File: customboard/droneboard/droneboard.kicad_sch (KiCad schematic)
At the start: 49 parts, among them J1 Conn_01x04, J2 USB_B_Micro, J3 Conn_01x05_Pin, J4 Conn_01x02_Pin, SW1 SW_Push, SW2 SW_Push, U1 STM32F411CEUx, U3 L78M05CDT, U4 ICM-42688-P, U5 LDK130M33R, U6 LDK130M33R, Y2 CSTNE20M0V53Z000R0

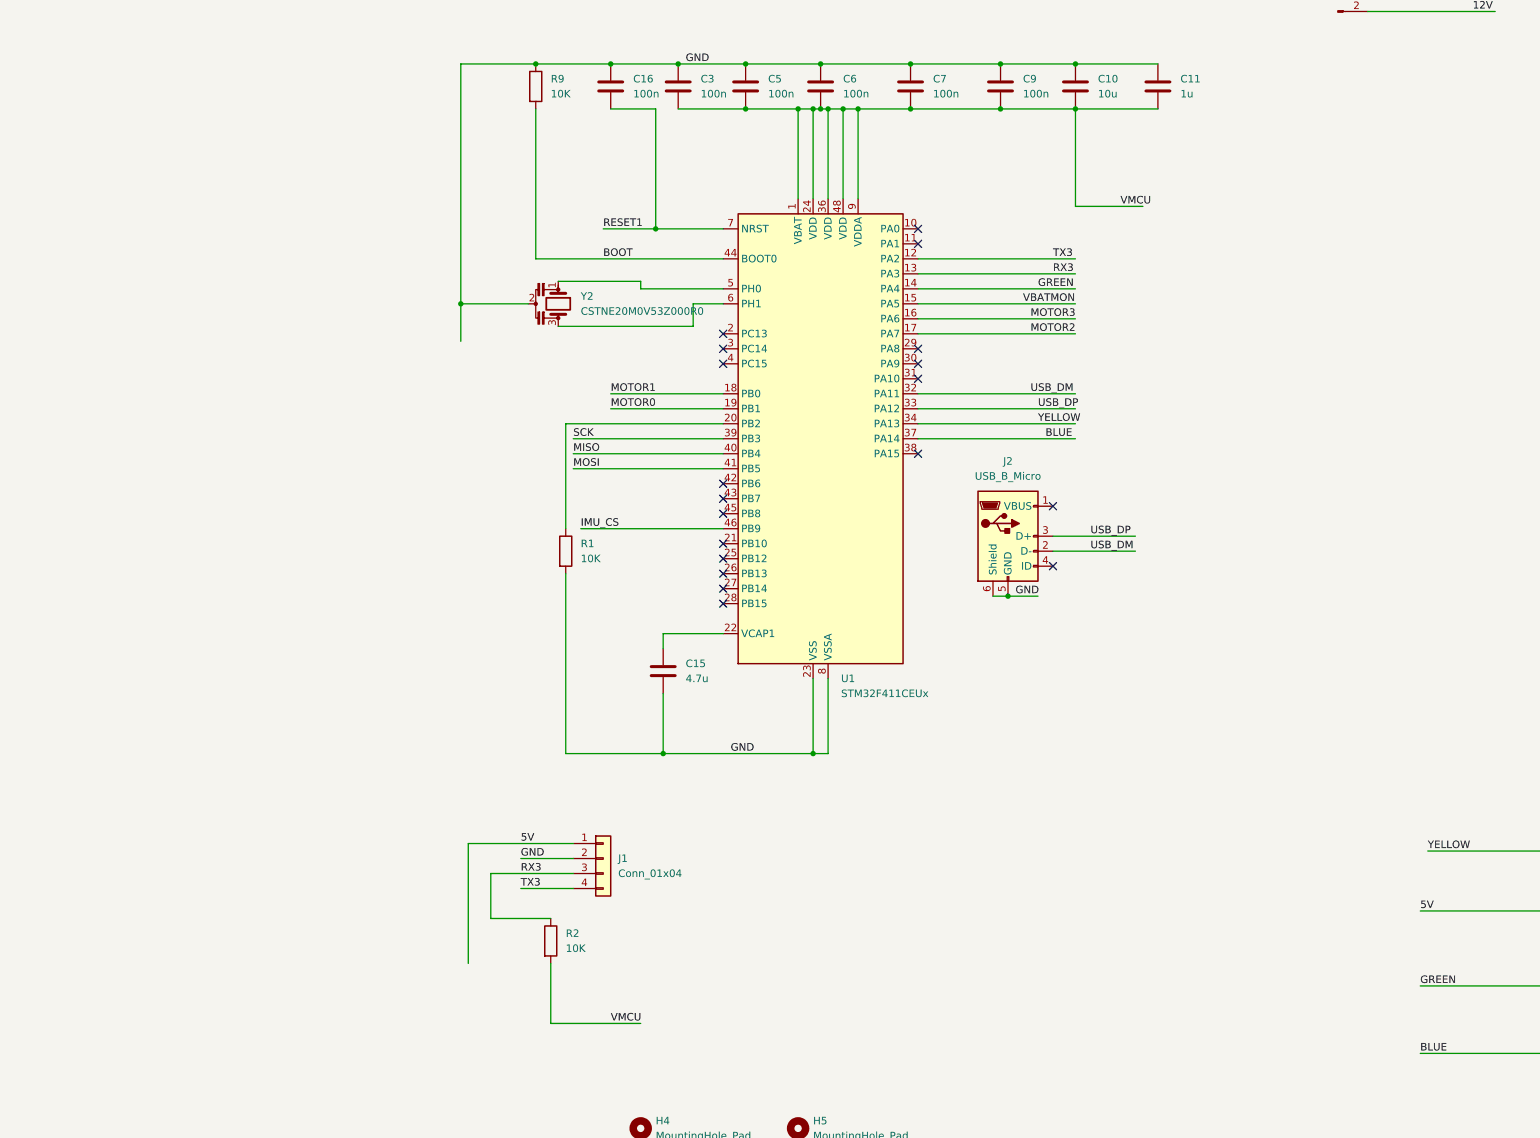
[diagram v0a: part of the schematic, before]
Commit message: h7 initial
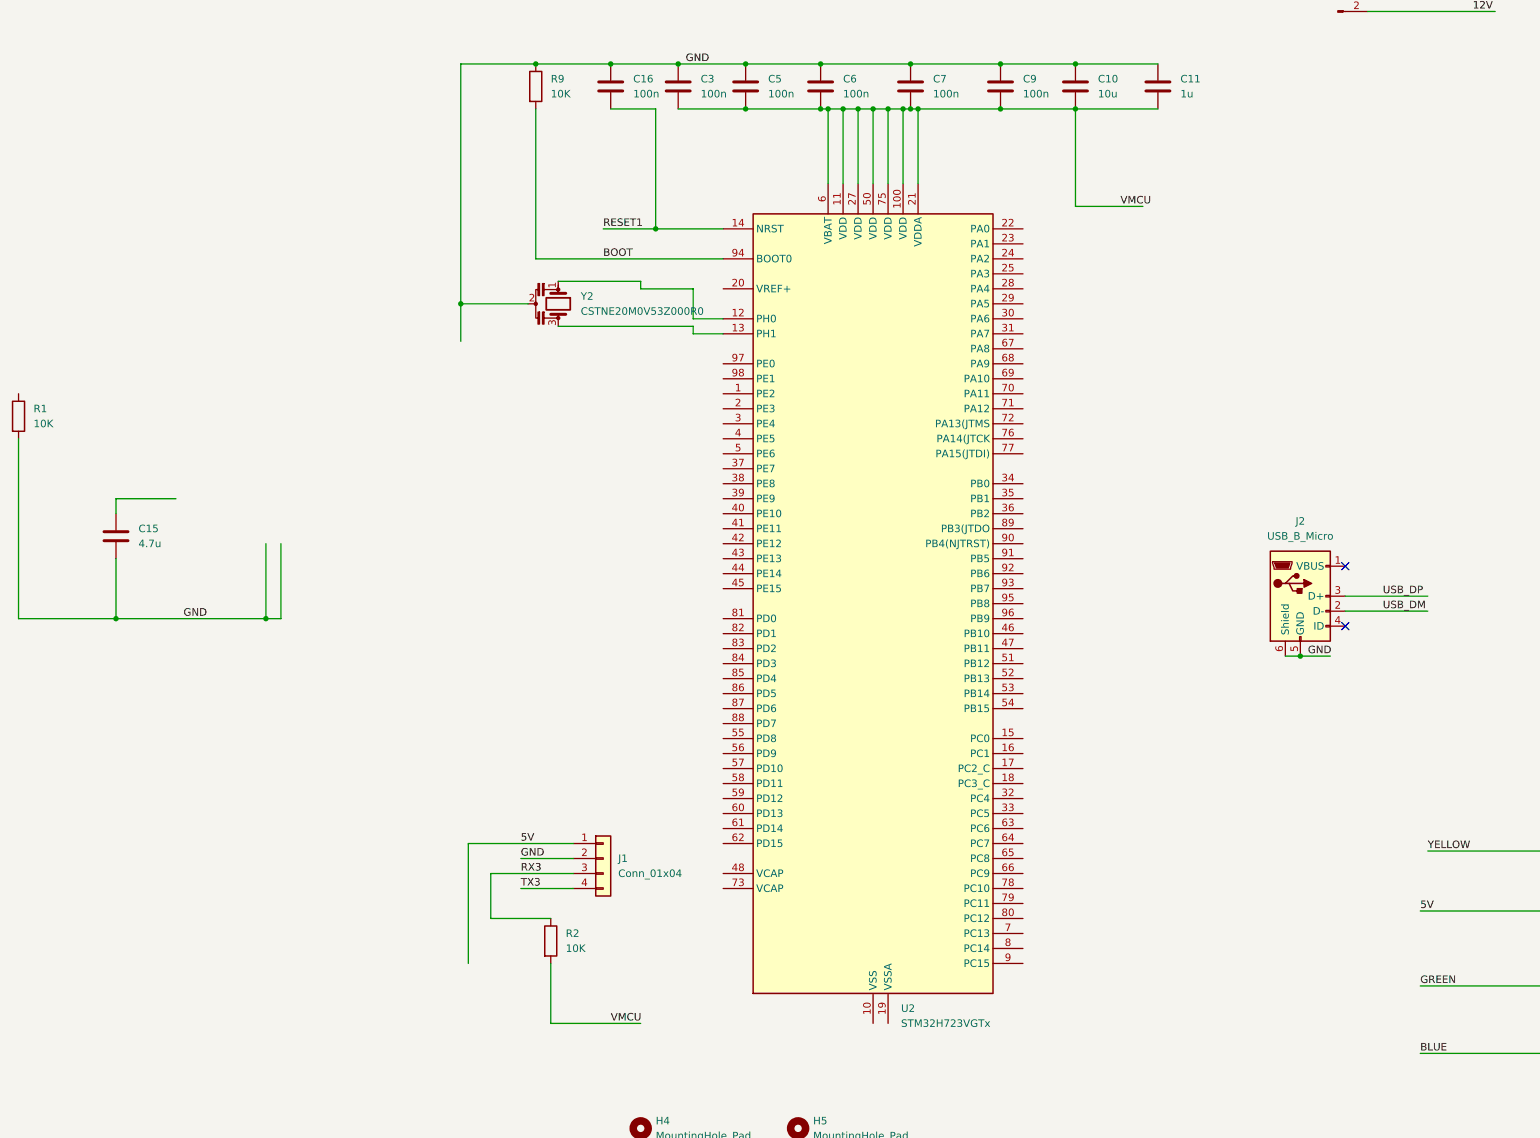
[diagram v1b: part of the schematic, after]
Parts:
- removed U1: STM32F411CEUx, Package_DFN_QFN:QFN-48-1EP_7x7mm_P0.5mm_EP5.6x5.6mm, symbol MCU_ST_STM32F4:STM32F411CEUx
- added U2: STM32H723VGTx, Package_QFP:LQFP-100_14x14mm_P0.5mm, symbol MCU_ST_STM32H7:STM32H723VGTx
- J4: footprint Connector_JST:JST_XH_B2B-XH-A_1x02_P2.50mm_Vertical -> Connector_PinHeader_1.27mm:PinHeader_1x02_P1.27mm_Vertical
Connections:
- net BOOT: now also U2.94 (BOOT0)
- net RESET1: now also U2.14 (NRST)
- net VMCU: now also U2.100 (VDD), U2.11 (VDD), U2.21 (VDDA), U2.27 (VDD), U2.50 (VDD), U2.6 (VBAT), U2.75 (VDD)
- net at Y2.1: now also U2.12 (PH0)
- net at Y2.3: now also U2.13 (PH1)
- new net: U2.10 (VSS), U2.26 (VSS), U2.49 (VSS), U2.74 (VSS), U2.99 (VSS)
- no-connect marks 20 -> 3
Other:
- moved on the sheet: C15, J2, R1
